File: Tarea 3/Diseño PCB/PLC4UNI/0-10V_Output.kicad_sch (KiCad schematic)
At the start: 8 parts, among them U16 GP8201S-TC50-EW

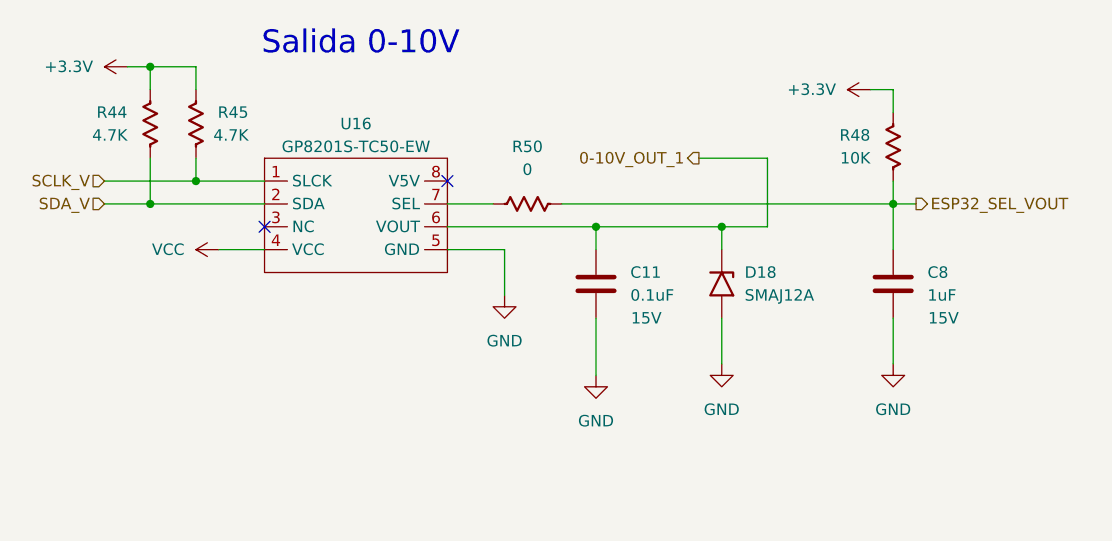
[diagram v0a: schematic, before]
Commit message: Tarea 3
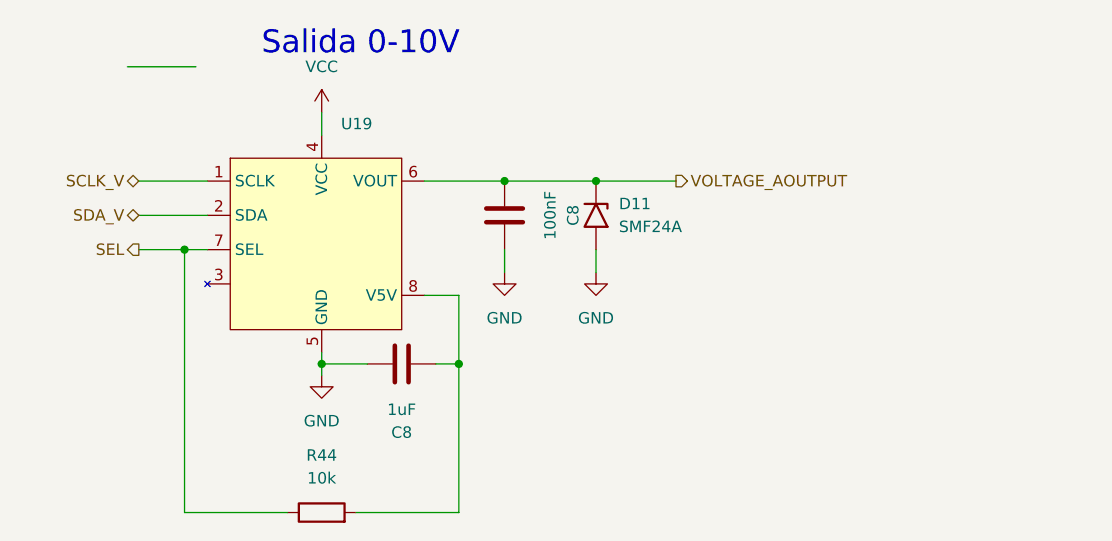
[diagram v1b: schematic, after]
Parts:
- removed C11: 0.1uF, PCM_Capacitor_SMD_AKL:C_0603_1608Metric, symbol PCM_Capacitor_US_AKL:C_0603
- removed C8: 1uF, PCM_Capacitor_SMD_AKL:C_0603_1608Metric, symbol PCM_Capacitor_US_AKL:C_0603
- removed D18: SMAJ12A, Diode_SMD:D_SMA, symbol Diode:SMAJ12A
- removed R44, R45: 4.7K, PCM_Resistor_SMD_AKL:R_0603_1608Metric, symbol PCM_Resistor_US_AKL:R_0603
- removed R48: 10K, PCM_Resistor_SMD_AKL:R_0603_1608Metric, symbol PCM_Resistor_US_AKL:R_0603
- removed R50: 0, PCM_Resistor_SMD_AKL:R_0603_1608Metric, symbol PCM_Resistor_US_AKL:R_0603
- removed U16: GP8201S-TC50-EW, Package_SO:SSOP-8_3.95x5.21x3.27mm_P1.27mm, symbol New_Library:GP8201S-TC50-EW
- added C8: 1uF, Capacitor_SMD:C_0805_2012Metric_Pad1.18x1.45mm_HandSolder, symbol Device:C
- added C8: 100nF, Capacitor_SMD:C_0805_2012Metric, symbol Device:C
- added D11: SMF24A, Diode_SMD:D_SMF, symbol Diode:SMF24A
- added R44: 10k, Resistor_SMD:R_0603_1608Metric, symbol Device:R
- added U19: ~, Package_SO:SOIC-8_5.3x5.3mm_P1.27mm, symbol Riqi_Parts:GP8201S
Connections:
- net GND: now also C8.1, C8.1, D11.2 (A2), U19.5 (GND)
- net SCLK_V: now also U19.1 (SCLK)
- net SDA_V: now also U19.2 (SDA)
- net VCC: now also U19.4 (VCC)
- new net: C8.2, R44.2, U19.8 (V5V)
- new net SEL: R44.1, U19.7 (SEL)
- new net VOLTAGE_AOUTPUT: C8.2, D11.1 (A1), U19.6 (VOUT)
- no-connect marks 2 -> 0
